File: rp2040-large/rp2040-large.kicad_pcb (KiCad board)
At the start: 2 copper layers, 21.3 x 51.6 mm, 30 parts, among them P1 USB2.0_C_12pin, P2 20Pin, P3 20Pin, SW1 SW_Push, U1 RP2040, U2 W25Q128JVS, U3 AZ1117-3.3, Y1 Crystal_GND24

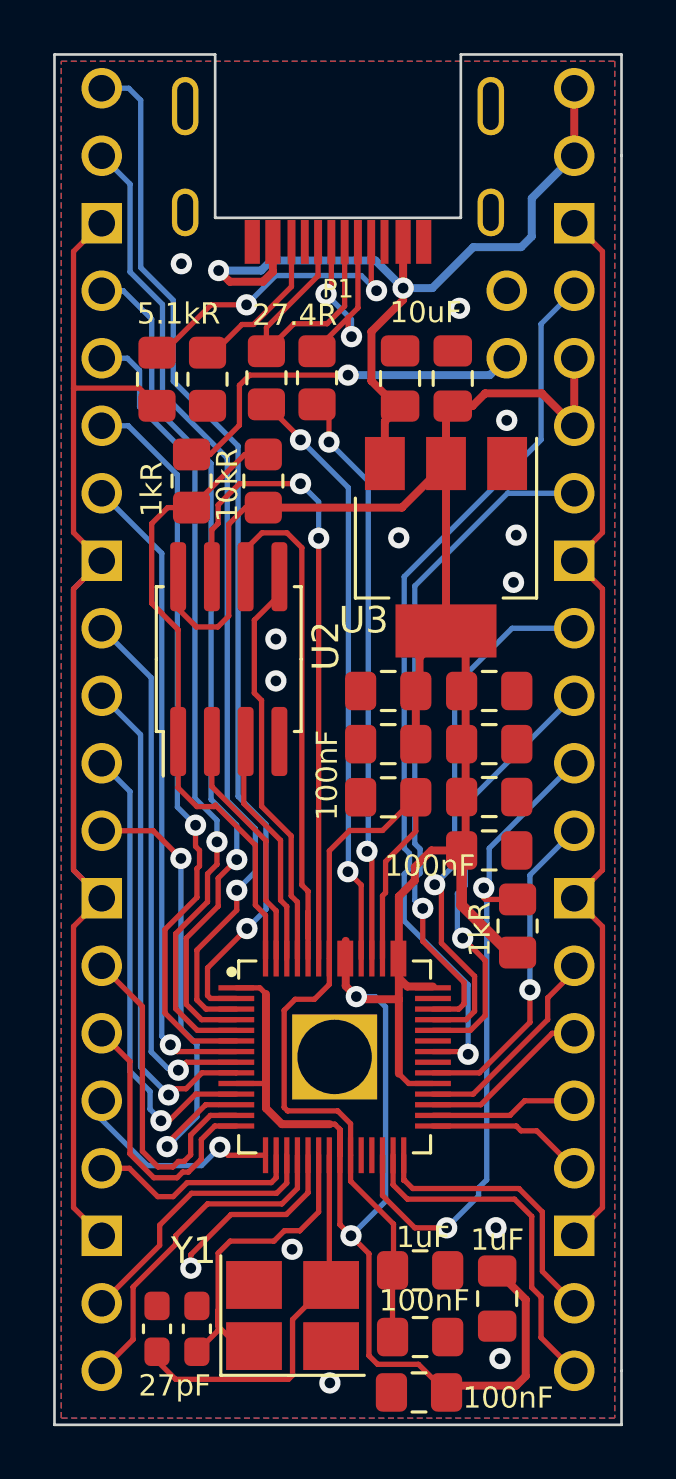
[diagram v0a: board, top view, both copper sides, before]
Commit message: rp2040-large v1.4.0
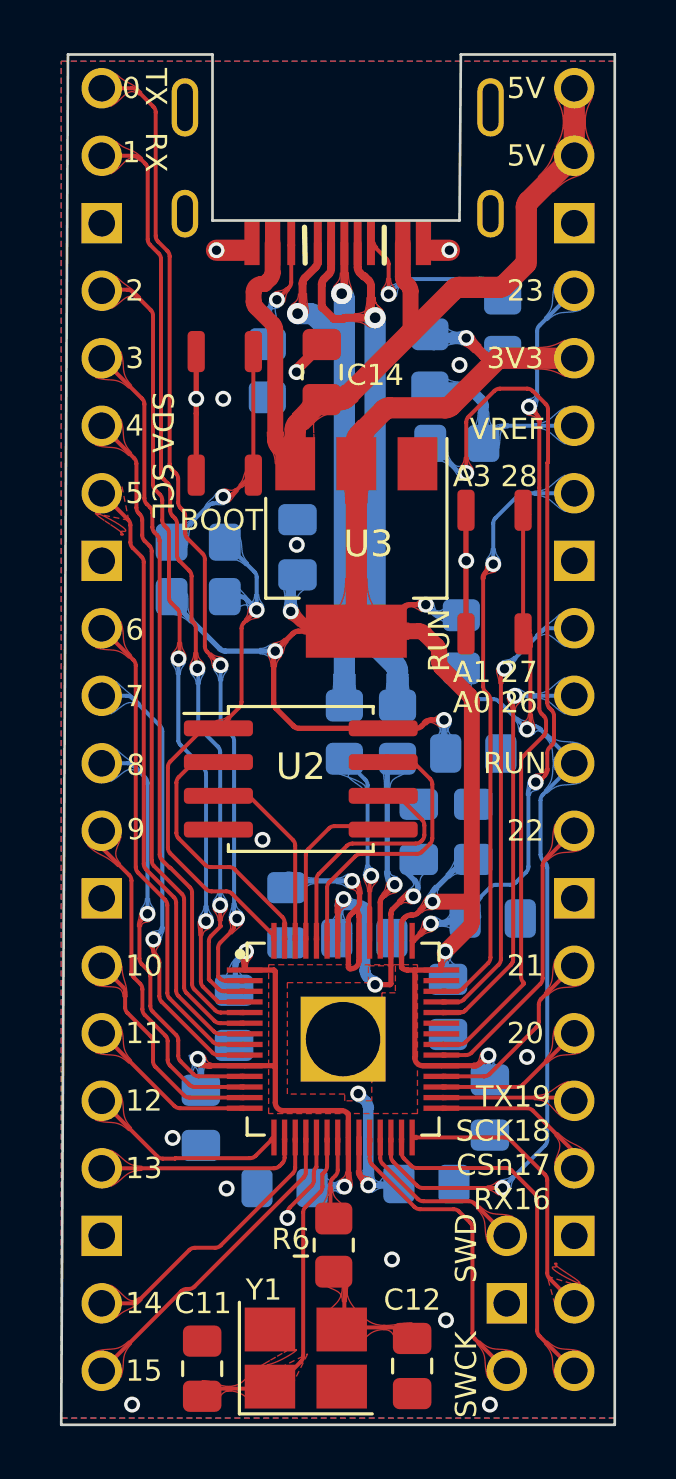
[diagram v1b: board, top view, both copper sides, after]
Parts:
- removed P1: USB2.0_C_12pin, rp2040-dev-board:USB-C-12-Pin-MidMount-ali-v2
- added C16: 100nF, rp2040-dev-board:Capacitor_0805_2012, B.Cu at (116.1, 74.4)
- added J1: USB2.0_C_v3, rp2040-dev-board:USB-C-12-Pin-MidMount-ali-v4, F.Cu at (118.1, 38.9)
- added J2: SWD, rp2040-dev-board:SWD_PIN, F.Cu at (124.5, 78.7)
- added R10: 1R, rp2040-dev-board:Register_0805_2012, B.Cu at (122.7, 46.5)
- added R8: 10kR, rp2040-dev-board:Register_0805_2012, B.Cu at (112.8, 52.0)
- added R9: 200R, rp2040-dev-board:Register_0805_2012, B.Cu at (121.7, 43.2)
- added SW2: SW_Push, rp2040-dev-board:SKRPABE010, F.Cu at (124.0, 51.2)
- C1, C10, C13, C15, C2, C3, C4, C5, C6, C7, C8, R1, R2, R3, R4, R5, R7: moved to B.Cu
- C11, C12: footprint rp2040-dev-board:Capacitor_0603_1608 -> rp2040-dev-board:Capacitor_0805_2012
- C9: value 100nF -> 1uF; moved to B.Cu
- R6: value 10kR -> 1kR
- SW1: footprint rp2040-dev-board:2Pin -> rp2040-dev-board:SKRPABE010
- moved R6 28.9 mm to (118.0, 76.7)
- moved C3 16.5 mm to (121.2, 61.0), turned to 90 degrees
- moved C5 16.5 mm to (116.2, 64.1)
- moved C10 15.7 mm to (113.0, 71.8), turned to -90 degrees
- moved C4 15.7 mm to (114.2, 68.0), turned to -90 degrees
- moved C8 15.7 mm to (123.8, 71.4), turned to -90 degrees
- moved R2 13.7 mm to (120.5, 57.1)
- moved R1 13.7 mm to (118.5, 57.1)
- moved R5 13.0 mm to (124.2, 42.0)
- moved SW1 11.1 mm to (113.8, 45.3), turned to 90 degrees
- moved R7 11.1 mm to (122.8, 53.8), turned to 90 degrees
- moved C6 10.0 mm to (122.2, 67.6), turned to -90 degrees
- moved C12 9.72 mm to (120.9, 81.1), turned to 90 degrees
- moved C15 8.63 mm to (116.6, 50.3)
- moved C1 5.76 mm to (121.4, 74.2)
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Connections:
- C12 pad 2: XOUT -> Net-(C12-Pad2)
- C9 pad 1: +3V3 -> Net-(C9-Pad1)
- P3 pad 4: 24 -> 23
- P3 pad 6: +3V3 -> ADC_VREF
- R6 pad 1: QSPI_SS -> XOUT
- R6 pad 2: +3V3 -> Net-(C12-Pad2)
- U1 pad 24: unconnected-(U1-Pad24) -> Net-(J2-Pad1)
- U1 pad 25: unconnected-(U1-Pad25) -> Net-(J2-Pad3)
- U1 pad 35: unconnected-(U1-Pad35) -> 23
- U1 pad 36: 24 -> unconnected-(U1-Pad36)
- U1 pad 43: +3V3 -> Net-(C9-Pad1)
- Y1 pad 3: XOUT -> Net-(C12-Pad2)
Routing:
- net GND: track 105.8 -> 16.2 mm, vias 13 -> 17
- net 24: track 33.9 -> 0.00 mm, vias 1 -> 0
- net 23: track 0.00 -> 31.4 mm, vias 0 -> 1
- net Net-(C9-Pad1): track 0.00 -> 31.4 mm, vias 0 -> 3
- net USB_DM: track 9.56 -> 24.6 mm, vias 2 -> 1
- net Net-(R1-Pad1): track 22.3 -> 7.41 mm, vias 2 -> 1
- net Net-(R2-Pad1): track 21.7 -> 7.59 mm, vias 2 -> 1
- net QSPI_SD3: track 23.9 -> 11.1 mm, vias 2 -> 0
- net +1V1: track 32.4 -> 20.1 mm, vias 0 -> 5
- net Net-(J2-Pad1): track 0.00 -> 11.7 mm
- net USB_DP: track 11.0 -> 22.6 mm, vias 0 -> 2
- net XOUT: track 14.8 -> 3.17 mm
- net ~{RESET}: track 25.7 -> 36.9 mm
- net QSPI_CLK: track 19.7 -> 9.58 mm
- net QSPI_SD0: track 15.4 -> 7.44 mm
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- added copper zone on F.Cu, net +1V1
- added copper zone on F.Cu, net +3V3
- added copper zone on F.Cu, net 17
- added copper zone on F.Cu, net 5
- added copper zone on F.Cu, net XIN
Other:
- board size 21.3 x 51.6 mm -> 20.8 x 51.6 mm
- board text added: "0"
- board text added: "1"
- board text added: "10"
- board text added: "11"
- board text added: "12"
- board text added: "13"
- board text added: "14"
- board text added: "15"
- board text added: "16"
- board text added: "17"
- board text added: "18"
- board text added: "19"
- board text added: "2"
- board text added: "20"
- board text added: "21"
- board text added: "23"
- board text added: "26"
- board text added: "27"
- board text added: "28"
- board text added: "3"
- board text added: "4"
- board text added: "5"
- board text added: "6"
- board text added: "7"
- board text added: "8"
- board text added: "9"
- board text added: "@74th"
- board text added: "A0 26"
- board text added: "A1 27"
- board text added: "A3 28"
- board text added: "RP2040L"
- board text added: "RX"
- board text added: "SCL"
- board text added: "SDA"
- board text added: "SWCK"
- board text added: "SWD"
- board text added: "TX"
- board text added: "TX19 SCK18 CSn17 RX16"
- board text added: "VREF"
- board text added: "v1.4.0"
- board text removed: "16/S0RX I0SDA/U0TX"
- board text removed: "17/S0CSn I0SCL/U0RX"
- board text removed: "18/S0SCK I1SDA"
- board text removed: "19/S0TX I1SCL"
- board text removed: "20/I0SDA"
- board text removed: "21/I0SCL"
- board text removed: "26/ADC0 I1SDA"
- board text removed: "27/ADC1 I1SCL"
- board text removed: "28/ADC2"
- board text removed: "EN"
- board text removed: "RP2040Large"
- board text removed: "S0CSn/1 I0SCL/U0RX"
- board text removed: "S0CSn/5 I0SCL/U1RX"
- board text removed: "S0RX/0 I0SDA/U0TX"
- board text removed: "S0RX/4 I0SDA/U1TX"
- board text removed: "S0SCK/2 I1SDA"
- board text removed: "S0SCK/6 I1SDA"
- board text removed: "S0TX/3 I1SCL"
- board text removed: "S0TX/7 I1SCL"
- board text removed: "S1CSn/13 I0SCL/U0RX"
- board text removed: "S1CSn/9 I0SCL/U1RX"
- board text removed: "S1RX/12 I0SDA/U0TX"
- board text removed: "S1RX/8 I0SDA/U1TX"
- board text removed: "S1SCK/10 I1SDA"
- board text removed: "S1SCK/14 I1SDA"
- board text removed: "S1TX/11 I1SCL"
- board text removed: "S1TX/15 I1SCL"
- board text removed: "v1.0.2"
